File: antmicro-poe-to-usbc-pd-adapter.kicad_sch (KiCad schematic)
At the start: 2 parts

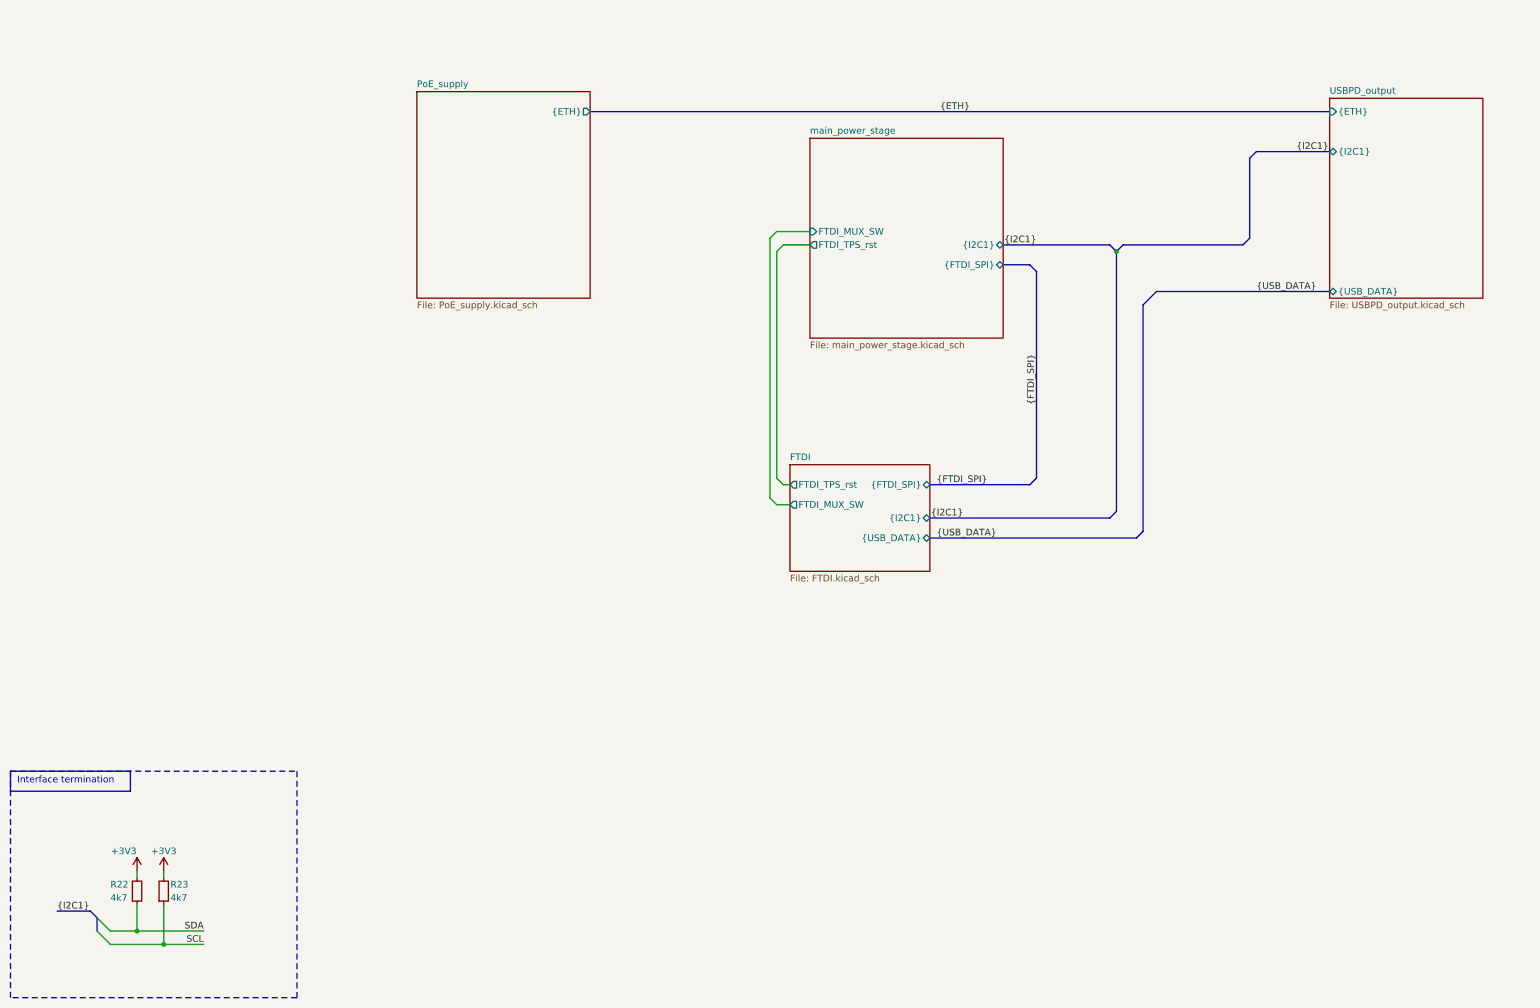
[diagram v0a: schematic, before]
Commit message: [#62623] Minor graphical changes
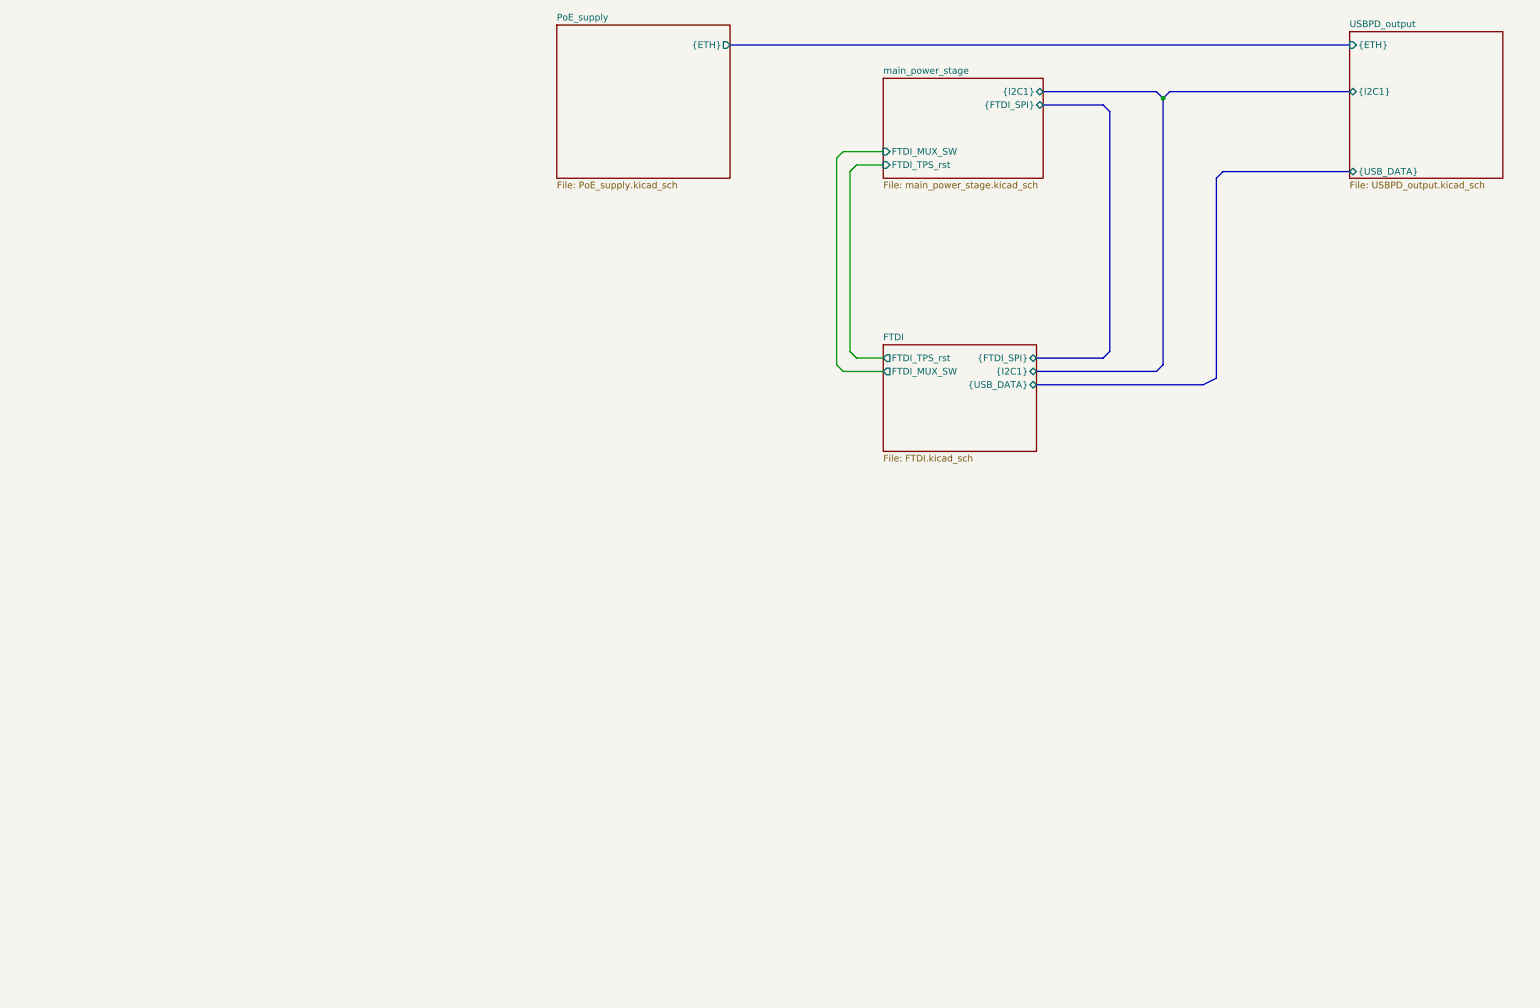
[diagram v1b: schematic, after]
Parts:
- removed R22, R23: R_4k7_0402, antmicro-footprints:R_0402_1005Metric, symbol antmicroResistors0402:R_4k7_0402
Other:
- note removed: "Interface termination"
